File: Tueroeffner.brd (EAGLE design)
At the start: 48.2 x 22.9 mm, 41 parts, among them IC1 NCP1117ST33T3G, IC3 M25PE20, K2 EC2-12TNU, Q1 2N7002CK, Q2 2N7002CK

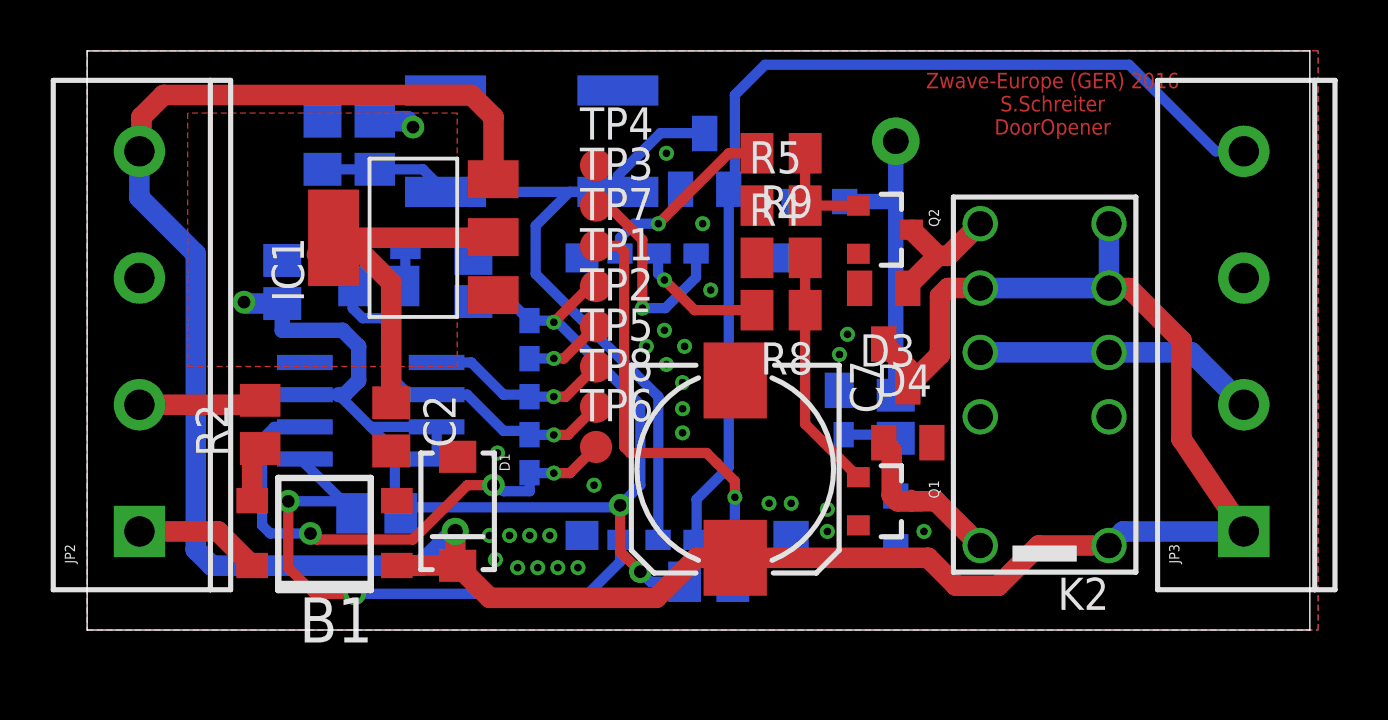
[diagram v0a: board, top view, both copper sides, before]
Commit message: Clean Up
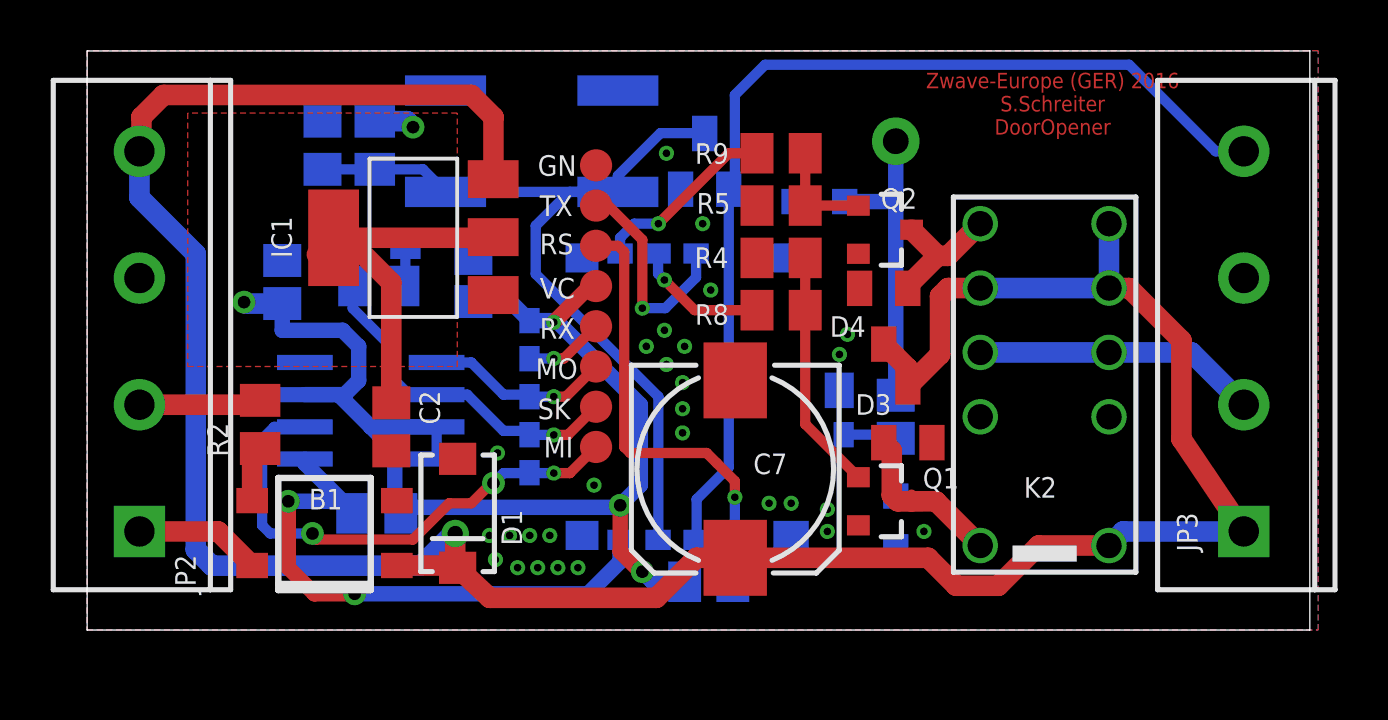
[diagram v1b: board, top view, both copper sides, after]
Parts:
- moved D1 0.08 mm to (13.0, 3.33)
- renumbered TP1 to VC, TP2 to RX, TP3 to TX, TP4 to GN, TP5 to MO, TP6 to MI, TP7 to RS, TP8 to SK
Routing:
- net MISO: track 20.8 -> 20.3 mm
